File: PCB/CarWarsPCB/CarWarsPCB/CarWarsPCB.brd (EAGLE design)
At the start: 66 x 56.8 mm, 21 parts, among them J1 MAGJACK, Q1 220mA/50V/3.5Ω, Q2 220mA/50V/3.5Ω

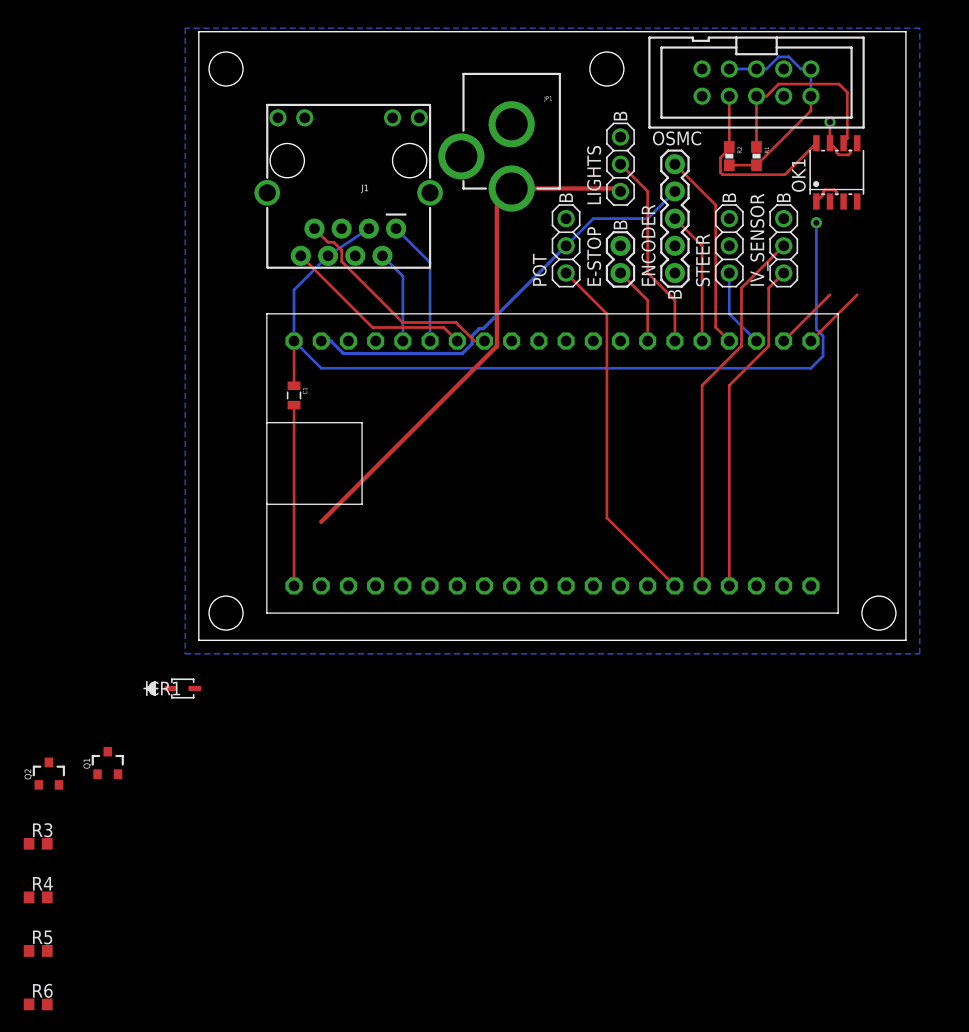
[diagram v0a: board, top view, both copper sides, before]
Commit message: post review
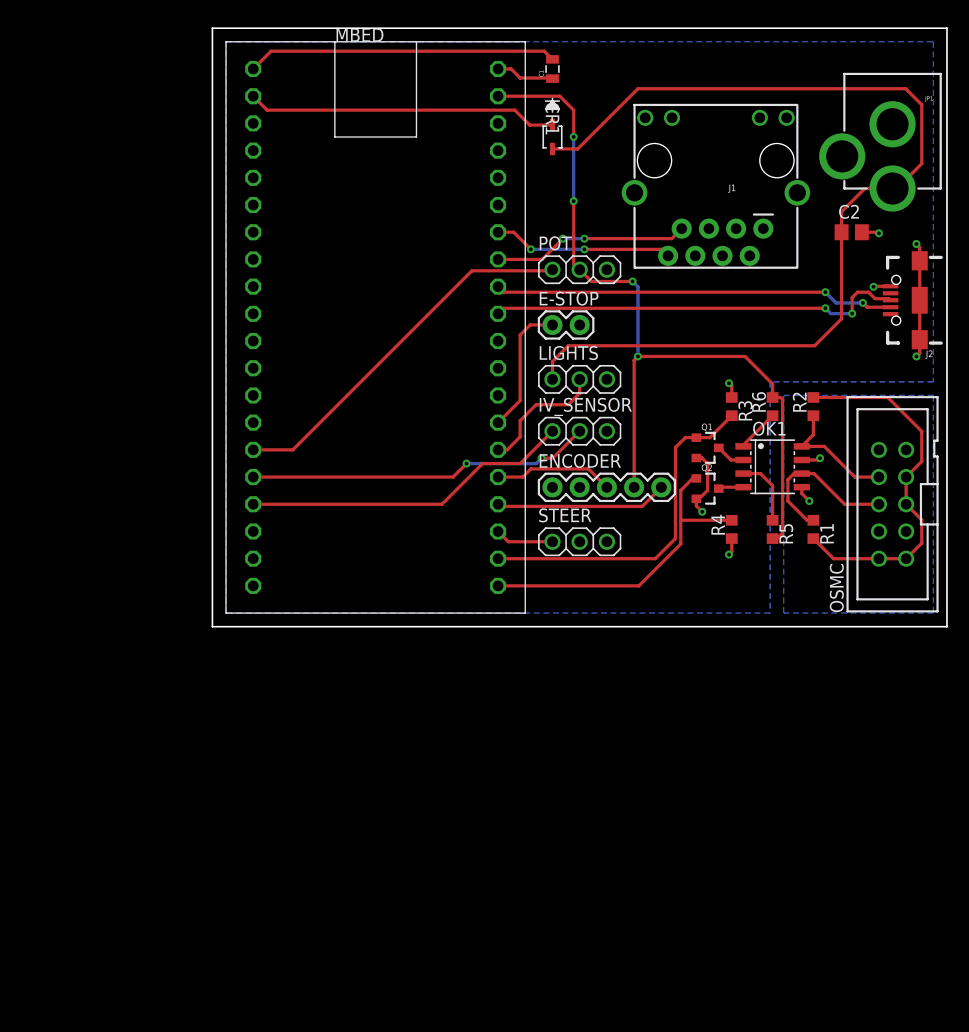
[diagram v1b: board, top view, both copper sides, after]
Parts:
- added C2: (no value), rcl:C0805
- added J2: (no value), SparkFun-Connectors:USB-B-MICRO-SMD
- C1: value 100nF -> 0.1uF
- R1, R2: device SparkFun-Resistors:0603-RES -> rcl:R0603
- R5, R6: value 10K -> 62
- moved R6 88.4 mm to (53.6, 21.8), turned to 90 degrees
- moved R5 79.1 mm to (53.6, 10.3), turned to 270 degrees
- moved R3 76.6 mm to (49.8, 21.8), turned to 270 degrees
- moved R4 73.3 mm to (49.8, 10.3), turned to 90 degrees
- moved Q2 67.0 mm to (47.5, 14.2), turned to 270 degrees
- moved Q1 63.2 mm to (47.5, 18.0), turned to 270 degrees
- moved CR1 62.0 mm to (33.0, 47.0), turned to 270 degrees
- moved OSMC 41.4 mm to (64.8, 12.7), turned to 90 degrees
- moved C1 38.9 mm to (33.0, 53.3), turned to 90 degrees
- moved JP1 35.6 mm to (64.8, 55.9)
- moved R1 35.3 mm to (57.4, 10.3)
- moved J1 34.3 mm to (55.9, 55.9)
- moved STEER 31.0 mm to (35.6, 9.20), turned to 0 degrees
- moved OK1 28.1 mm to (53.6, 16.2), turned to 270 degrees
- moved IV_SENSOR 25.7 mm to (35.6, 19.5), turned to 0 degrees
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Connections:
- new net N$4: OK1.3, R5.1
- new net N$5: OK1.1, R6.1
- new net N$7: J2.D-, MBED.32
- new net N$8: J2.D+, MBED.31
- new net VBUS: J2.VBUS
- net +3V3: no longer Q1.1, Q2.1, R3.2, R4.2
- net +5V: no longer OK1.1, OK1.3
- net DRIVE_DIR_3V3: now also Q1.1, R3.2; no longer Q1.2, R3.1
- net DRIVE_PWM_3V3: now also Q2.1, R4.2; no longer Q2.2, R4.1
- net GND: now also C2.2, J2.GND, J2.SHIELD1, J2.SHIELD2, J2.SHIELD3, Q1.2, Q2.2, R3.1, R4.1
- net N$2: no longer R5.1
- net N$3: no longer R6.1
- net VCC: now also C2.1
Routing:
- net +3V3: track 81.7 -> 5.45 mm, vias 1 -> 0
- net VCC: track 48.8 -> 92.6 mm
- net N$8: track 0.00 -> 39.1 mm, vias 0 -> 2
- net N$7: track 0.00 -> 37.0 mm, vias 0 -> 2
- net GND: track 16.9 -> 52.6 mm, vias 0 -> 7
- net +5V: track 43.1 -> 77.2 mm, vias 0 -> 4
- net N$1: track 0.00 -> 29.1 mm
- net DRIVE_DIR_3V3: track 6.11 -> 32.4 mm
- net DRIVE_PWM_3V3: track 6.11 -> 30.4 mm
- net +12V: track 22.2 -> 34.6 mm
- net ETH_RD+: track 11.8 -> 0.00 mm
- net ETH_RD-: track 8.74 -> 0.00 mm
- net NEOPIXEL_CONTROL: track 18.6 -> 12.0 mm
- net N$4: track 0.00 -> 6.42 mm
- net DRIVE_DIR_12V: track 17.7 -> 11.7 mm
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- added copper zone on layer 16, net DGND
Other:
- board size 66 x 56.8 mm -> 68.6 x 55.9 mm
- board text removed: "B"
